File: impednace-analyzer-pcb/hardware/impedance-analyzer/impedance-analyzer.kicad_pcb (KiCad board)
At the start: 2 copper layers, 126.3 x 60.1 mm, 16 parts, among them J1 AD9833, J10 Conn_01x08, J11 Conn_01x08, J2 ADS1256_SPI, J3 ADS1256_AIN, J4 UNO_POWER, J5 UNO_ANALOG, J6 UNO_DIGITAL_LOW, J7 UNO_DIGITAL_HIGH, J8 Conn_01x08, J9 Conn_01x08, U1 CD74HC4067M

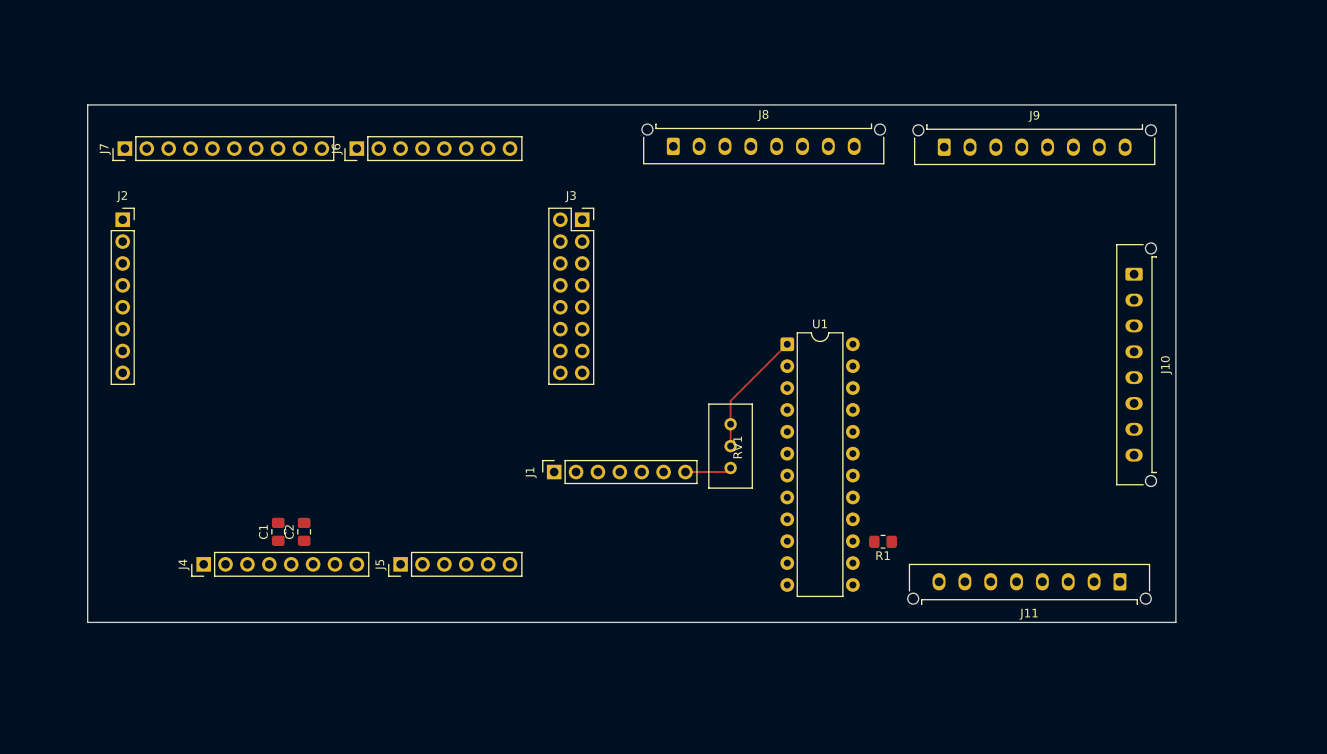
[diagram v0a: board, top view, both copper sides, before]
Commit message: finished routing, waiting review
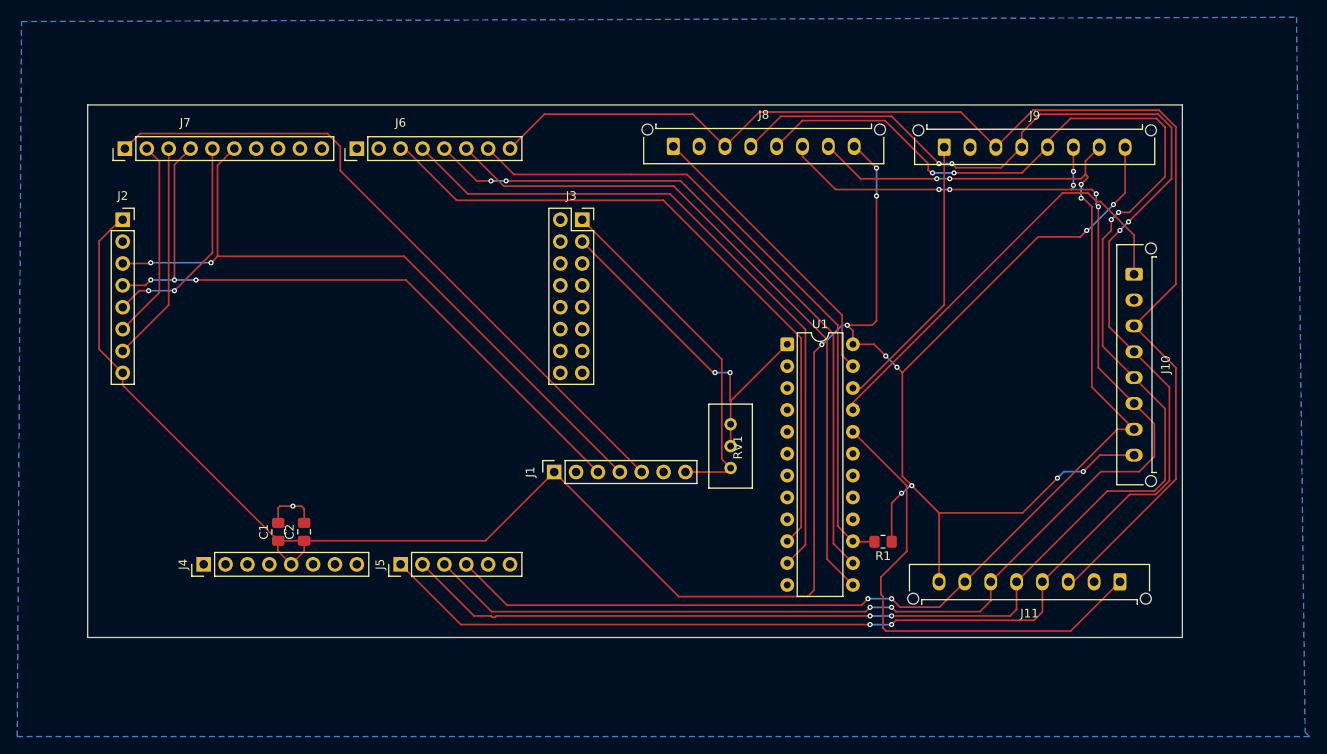
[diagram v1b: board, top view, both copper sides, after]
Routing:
- net +5V: track 0.00 -> 292.0 mm, vias 0 -> 12
- net DB_S1: track 0.00 -> 205.0 mm, vias 0 -> 6
- net DB_S2: track 0.00 -> 197.7 mm, vias 0 -> 6
- net DB_S3: track 0.00 -> 169.2 mm, vias 0 -> 8
- net DB_EN: track 0.00 -> 157.7 mm, vias 0 -> 6
- net DB_S0: track 0.00 -> 148.8 mm
- net SCLK: track 0.00 -> 81.7 mm, vias 0 -> 2
- net MB_S2: track 0.00 -> 81.6 mm, vias 0 -> 2
- net MB_S1: track 0.00 -> 81.1 mm
- net MB_S3: track 0.00 -> 80.8 mm
- net SDATA: track 0.00 -> 80.7 mm, vias 0 -> 3
- net MB_S0: track 0.00 -> 79.9 mm
- net FSYNC: track 0.00 -> 78.6 mm
- net MB_EN: track 0.00 -> 77.4 mm
- net JACK3_SIG: track 0.00 -> 56.7 mm
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- added copper zone on B.Cu, net GND
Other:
- board size 126.3 x 60.1 mm -> 127.1 x 61.8 mm
